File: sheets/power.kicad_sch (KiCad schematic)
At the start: 36 parts, among them J3 USB_C_Receptacle_USB2.0_16P, SW3 SW_SPDT, SW4 SW_SPDT, U4 LMR51430XFDDCR, U6 USBLC6-2P6, U8 TPS54620RGYR, U9 AMS1117-3.3

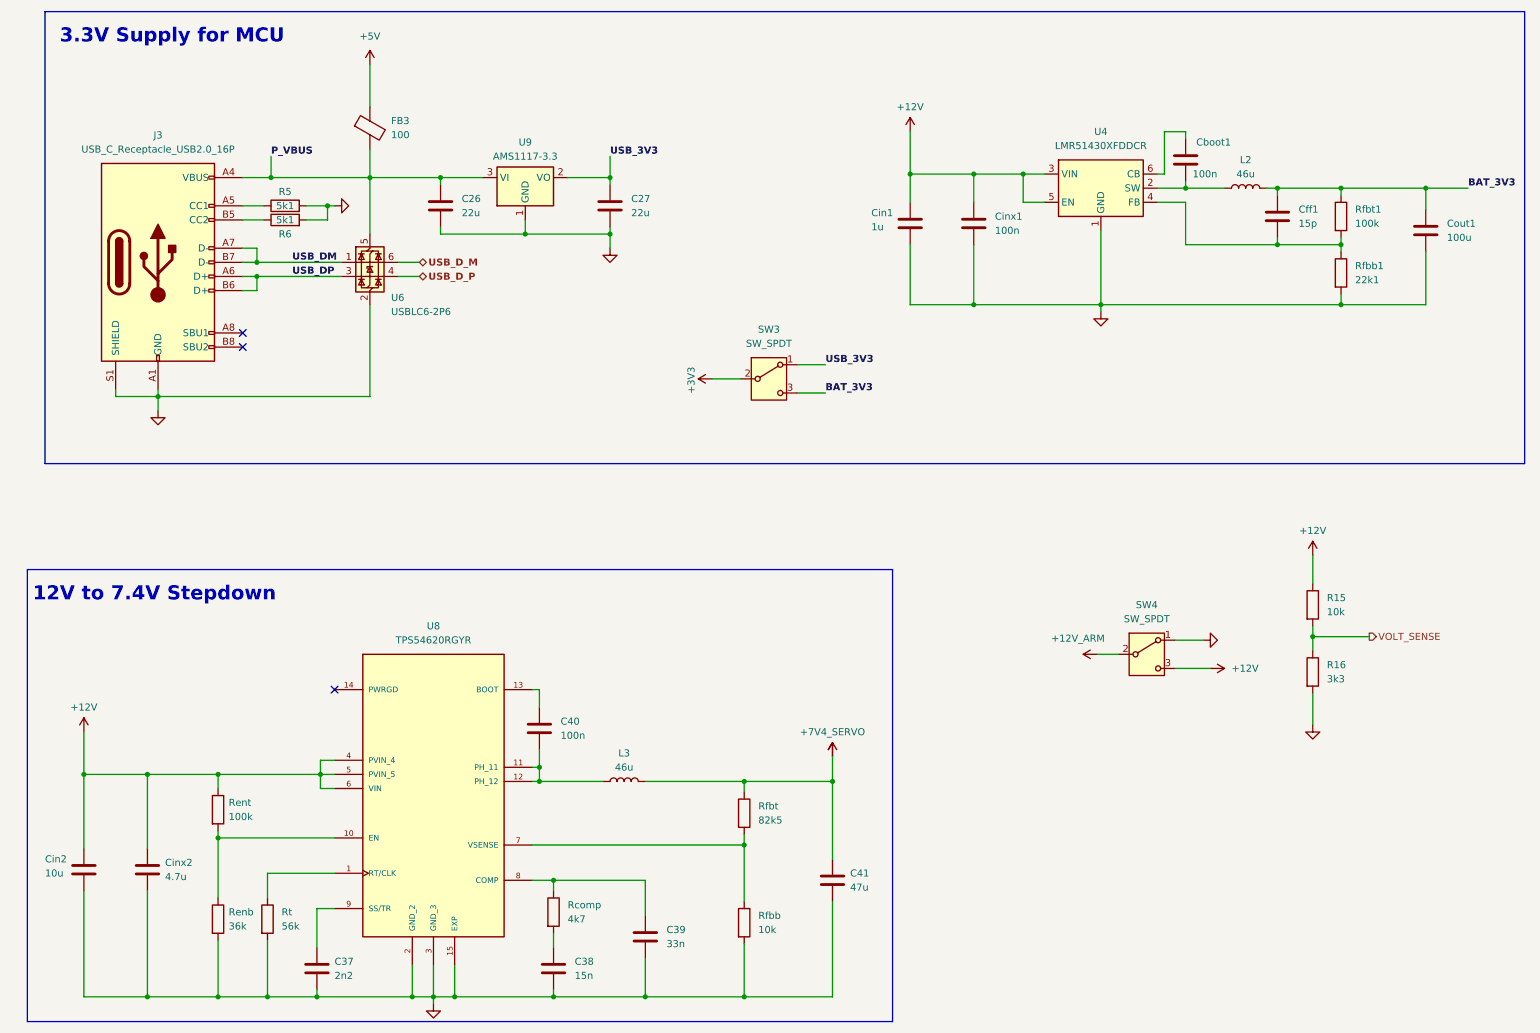
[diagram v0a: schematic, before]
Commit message: Rev1 schematic done
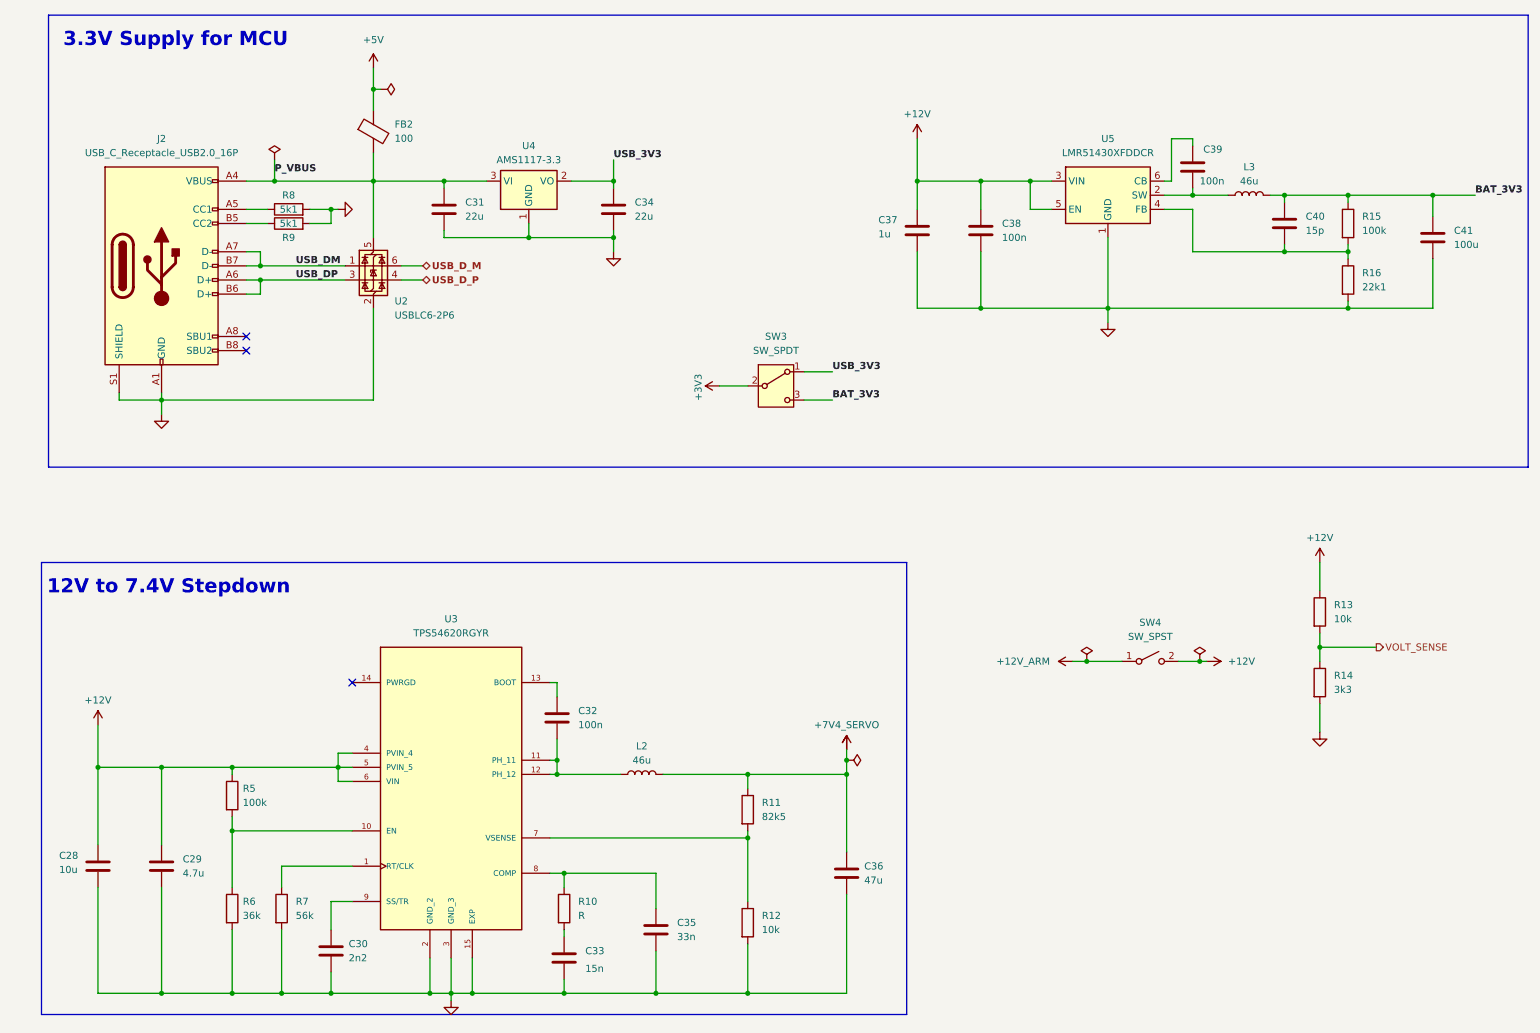
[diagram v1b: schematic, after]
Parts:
- removed Rcomp: 4k7, symbol Device:R
- removed SW4: SW_SPDT, symbol Switch:SW_SPDT
- removed U8: TPS54620RGYR, TPS54620RGYR:QFN50P350X350X100-15N, symbol aerolotl_custom:TPS54620RGYR
- added R10: R, symbol Device:R
- added SW4: SW_SPST, symbol Switch:SW_SPST
- added U3: TPS54620RGYR, TPS54620RGYR:QFN50P350X350X100-15N, symbol aerolotl_custom:TPS54620RGYR
- renumbered Cin2 to C28, Cinx2 to C29, C37 to C30, C26 to C31, C40 to C32, C38 to C33, C27 to C34, C39 to C35, C41 to C36, Cin1 to C37, Cinx1 to C38, Cboot1 to C39, Cff1 to C40, Cout1 to C41, FB3 to FB2, J3 to J2, L3 to L2, L2 to L3, Rfbt to R11, Rfbb to R12, R15 to R13, R16 to R14, Rfbt1 to R15, Rfbb1 to R16, Rent to R5, Renb to R6, Rt to R7, R5 to R8, R6 to R9, U6 to U2, U9 to U4, U4 to U5
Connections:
- net +12V: now also SW4.2 (B), U3.4 (PVIN_4), U3.5 (PVIN_5), U3.6 (VIN)
- net +12V_ARM: now also SW4.1 (A)
- net GND: now also U3.15 (EXP), U3.2 (GND_2), U3.3 (GND_3)
- net at C35.1: now also R10.1, U3.8 (COMP)
- net at C33.1: now also R10.2
- net at C32.1: now also U3.13 (BOOT)
- net at C32.2, L2.1: now also U3.11 (PH_11), U3.12 (PH_12)
- net at R5.2, R6.1: now also U3.10 (EN)
- net at R11.2, R12.1: now also U3.7 (VSENSE)
- net at C30.1: now also U3.9 (SS/TR)
- net at R7.1: now also U3.1 (RT/CLK)
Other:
- moved on the sheet: C28, C29, C30, C31, C32, C33, C34, C35, C36, C37, C38, C39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
